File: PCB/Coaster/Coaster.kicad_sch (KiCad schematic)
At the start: 84 parts, among them J1 Join, J2 Shelly, J3 USB-C, P1 TestPoint, P10 TestPoint, P11 TestPoint, P12 TestPoint, P13 TestPoint, P14 TestPoint, P15 TestPoint, P16 TestPoint, P17 TestPoint, P2 TestPoint, P5 TestPoint, P6 TestPoint, P7 TestPoint, P8 TestPoint, P9 TestPoint, T1 TestPoint, T10 TestPoint, T11 TestPoint, T12 TestPoint, T13 TestPoint, T14 TestPoint, T15 TestPoint, T16 TestPoint, T17 TestPoint, T2 TestPoint, T5 TestPoint, T6 TestPoint, T7 TestPoint, T8 TestPoint, T9 TestPoint, U1 ESP32-PICO-MINI-02, U2 LMR16006XDDCR, U3 QR

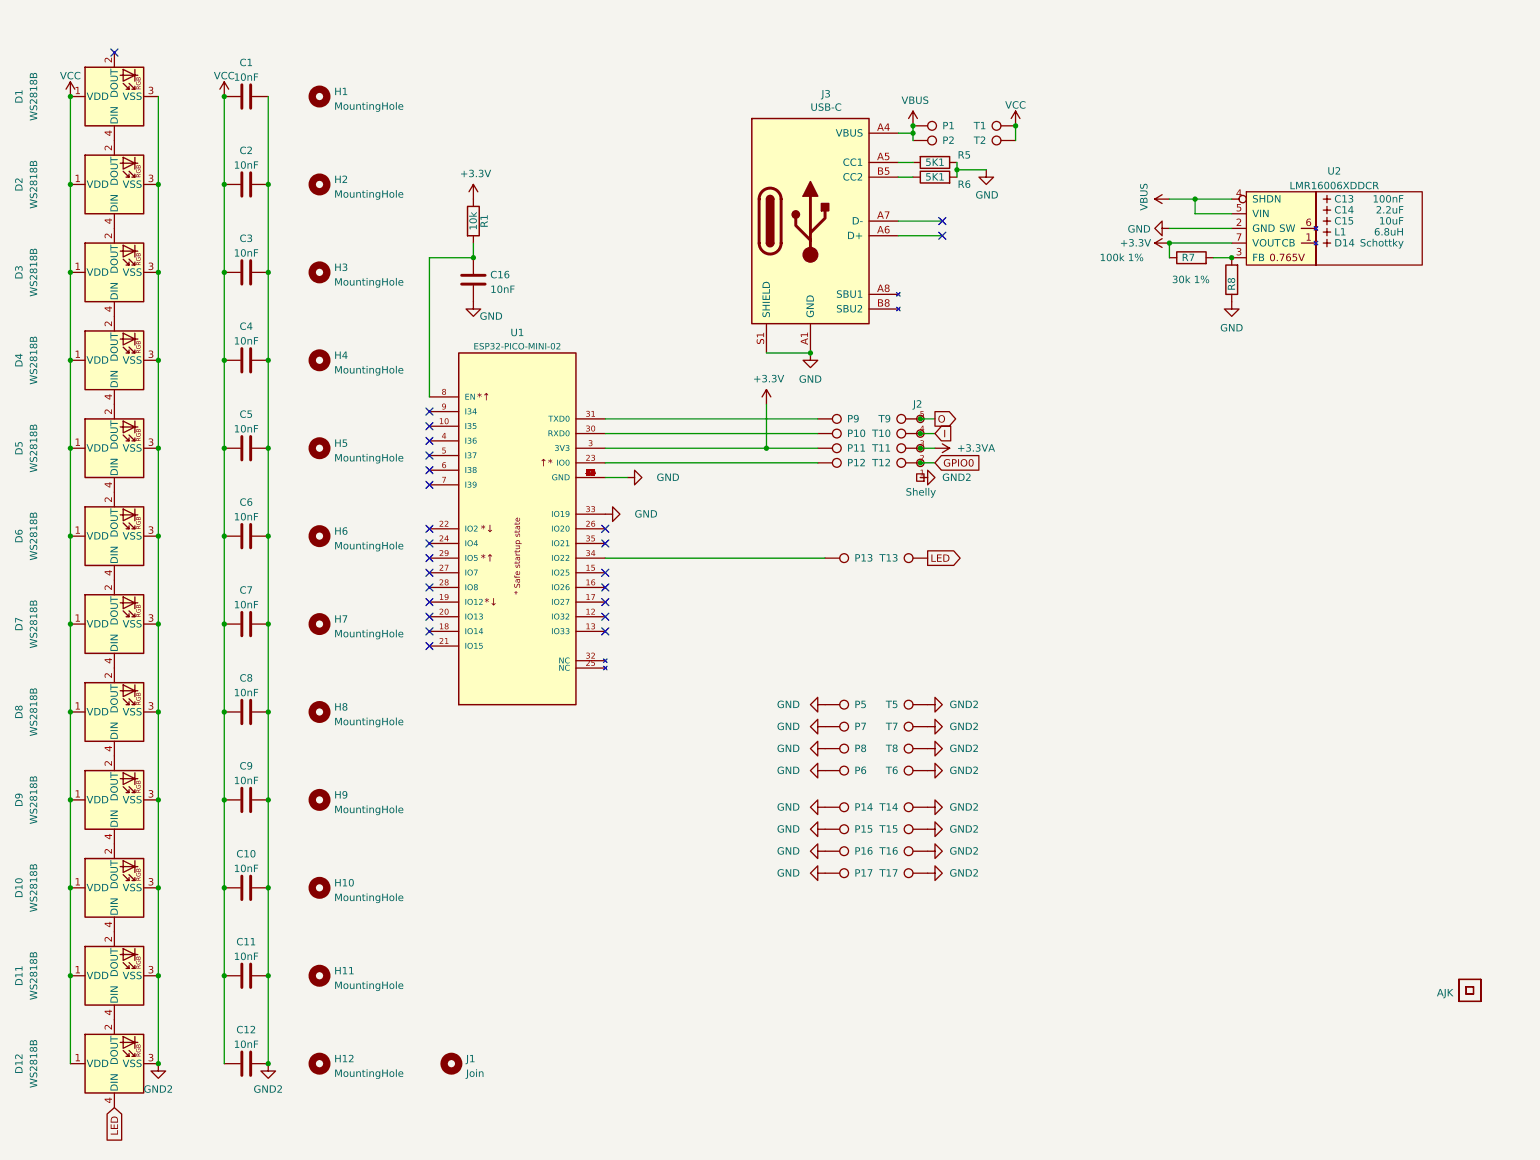
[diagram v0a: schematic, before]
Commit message: Much tidying
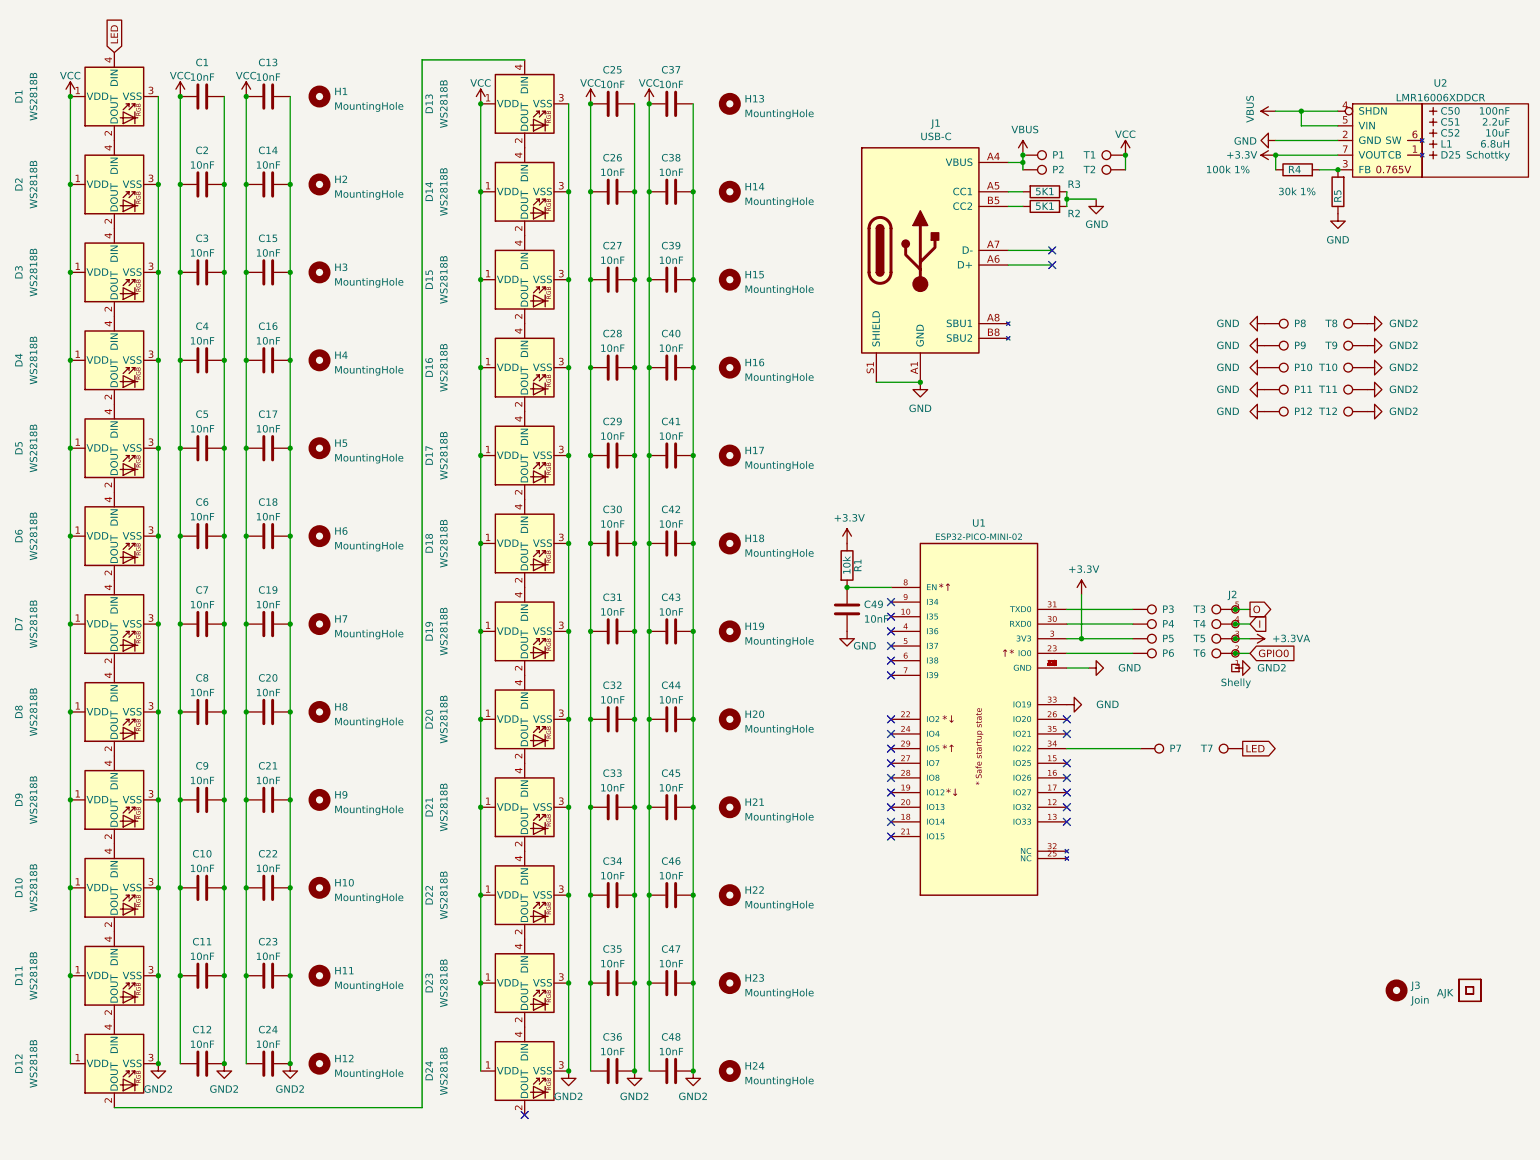
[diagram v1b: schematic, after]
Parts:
- removed P14, P15, P16, P17: TestPoint, RevK:PAD, symbol Connector:TestPoint
- removed T14, T15, T16, T17: TestPoint, RevK:PAD-LINK, symbol Connector:TestPoint
- added C13, C14, C15, C16, C17, C18, C19, C20, C21, C22, C23, C24, C25, C26, C27, C28, C29, C30, C31, C32, C33, C34, C35, C36, C37, C38, C39, C40, C41, C42, C43, C44, C45, C46, C47, C48: 10nF, RevK:C_0603, symbol Device:C
- added D13, D14, D15, D16, D17, D18, D19, D20, D21, D22, D23, D24: WS2818B, RevK:SMD2020, symbol LED:WS2812B
- added H13, H14, H15, H16, H17, H18, H19, H20, H21, H22, H23, H24: MountingHole, RevK:LEDHOLE, symbol Mechanical:MountingHole
- added P12: TestPoint, RevK:PAD, symbol Connector:TestPoint
- added T12: TestPoint, RevK:PAD-LINK, symbol Connector:TestPoint
- D1, D10, D11, D12, D2, D3, D4, D5, D6, D7, D8, D9: footprint RevK:SMD5050 -> RevK:SMD2020; LCSC Part # C114586 -> C784564
- renumbered C16 to C49, C13 to C50, C14 to C51, C15 to C52, D14 to D25, J3 to J1, J1 to J3, P8 to P10, P6 to P11, P9 to P3, P10 to P4, P11 to P5, P12 to P6, P13 to P7, P5 to P8, P7 to P9, R6 to R2, R5 to R3, R7 to R4, R8 to R5, T8 to T10, T6 to T11, T9 to T3, T10 to T4, T11 to T5, T12 to T6, T13 to T7, T5 to T8, T7 to T9
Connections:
- net GND: now also P12.1
- net GND2: now also C13.2, C14.2, C15.2, C16.2, C17.2, C18.2, C19.2, C20.2, C21.2, C22.2, C23.2, C24.2, C25.2, C26.2, C27.2, C28.2, C29.2, C30.2, C31.2, C32.2, C33.2, C34.2, C35.2, C36.2, C37.2, C38.2, C39.2, C40.2, C41.2, C42.2, C43.2, C44.2, C45.2, C46.2, C47.2, C48.2, D13.3 (VSS), D14.3 (VSS), D15.3 (VSS), D16.3 (VSS), D17.3 (VSS), D18.3 (VSS), D19.3 (VSS), D20.3 (VSS), D21.3 (VSS), D22.3 (VSS), D23.3 (VSS), D24.3 (VSS), T12.1
- net LED: now also D1.4 (DIN); no longer D12.4 (DIN)
- net VCC: now also C13.1, C14.1, C15.1, C16.1, C17.1, C18.1, C19.1, C20.1, C21.1, C22.1, C23.1, C24.1, C25.1, C26.1, C27.1, C28.1, C29.1, C30.1, C31.1, C32.1, C33.1, C34.1, C35.1, C36.1, C37.1, C38.1, C39.1, C40.1, C41.1, C42.1, C43.1, C44.1, C45.1, C46.1, C47.1, C48.1, D13.1 (VDD), D14.1 (VDD), D15.1 (VDD), D16.1 (VDD), D17.1 (VDD), D18.1 (VDD), D19.1 (VDD), D20.1 (VDD), D21.1 (VDD), D22.1 (VDD), D23.1 (VDD), D24.1 (VDD)
- net at D1.2 (DOUT): now also D2.4 (DIN)
- net at D2.2 (DOUT): now also D3.4 (DIN); no longer D1.4 (DIN)
- net at D11.4 (DIN): now also D10.2 (DOUT); no longer D12.2 (DOUT)
- net at D11.2 (DOUT): now also D12.4 (DIN); no longer D10.4 (DIN)
- net at D4.2 (DOUT): now also D5.4 (DIN); no longer D3.4 (DIN)
- net at D4.4 (DIN): now also D3.2 (DOUT); no longer D5.2 (DOUT)
- net at D8.4 (DIN): now also D7.2 (DOUT); no longer D9.2 (DOUT)
- net at D9.4 (DIN): now also D8.2 (DOUT); no longer D10.2 (DOUT)
- net at D6.2 (DOUT): now also D7.4 (DIN); no longer D5.4 (DIN)
- net at D6.4 (DIN): now also D5.2 (DOUT); no longer D7.2 (DOUT)
- new net: D15.2 (DOUT), D16.4 (DIN)
- new net: D14.2 (DOUT), D15.4 (DIN)
- new net: D23.2 (DOUT), D24.4 (DIN)
- new net: D12.2 (DOUT), D13.4 (DIN)
- new net: D20.2 (DOUT), D21.4 (DIN)
- new net: D19.2 (DOUT), D20.4 (DIN)
- new net: D13.2 (DOUT), D14.4 (DIN)
- new net: D16.2 (DOUT), D17.4 (DIN)
- new net: D18.2 (DOUT), D19.4 (DIN)
- new net: D17.2 (DOUT), D18.4 (DIN)
- new net: D10.4 (DIN), D9.2 (DOUT)
- new net: D21.2 (DOUT), D22.4 (DIN)
- new net: D22.2 (DOUT), D23.4 (DIN)
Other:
- moved on the sheet: C1, C10, C11, C12, C2, C3, C4, C49, C5, C50, C51, C52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
